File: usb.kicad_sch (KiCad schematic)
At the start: 8 parts, among them IC2 USB Hub, J2 2-Port USB, J3 2-Port USB

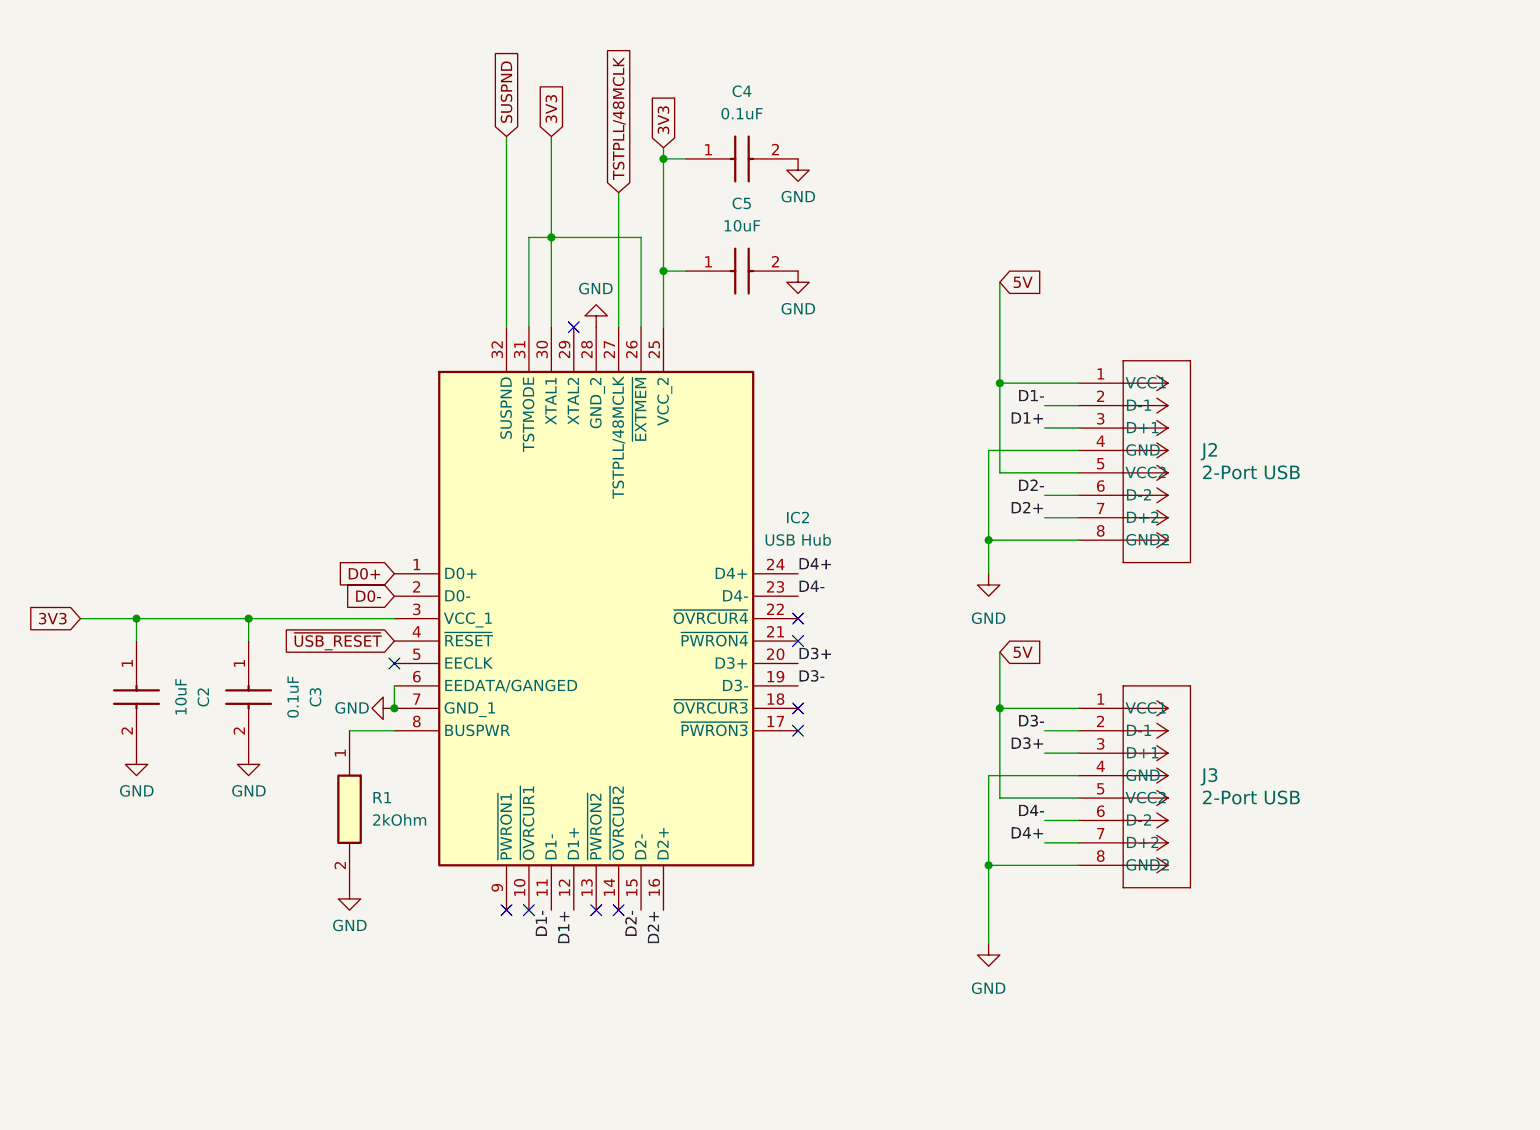
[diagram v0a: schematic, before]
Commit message: schematic fixes are done
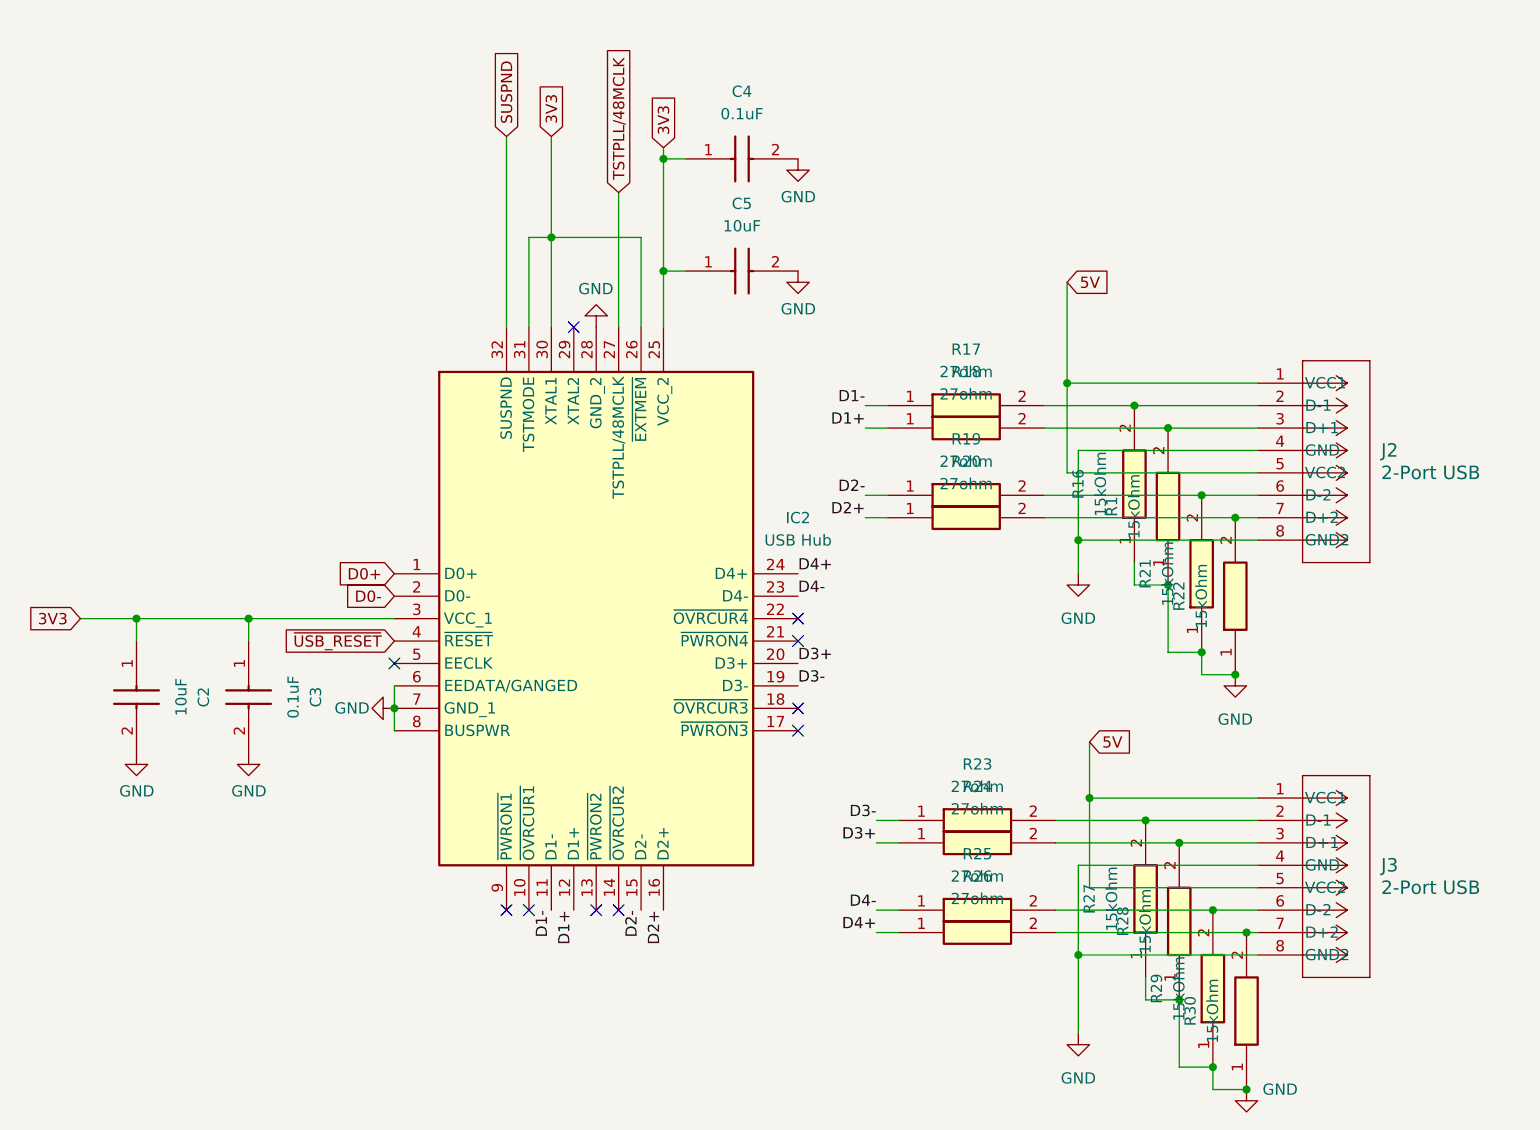
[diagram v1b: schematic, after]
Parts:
- added R16, R21, R22, R27, R28, R29, R30: 15kOhm, RESC2012X60N, symbol group127:Resistor
- added R17, R18, R19, R20, R23, R24, R25, R26: 27ohm, RESC2012X60N, symbol group127:Resistor
- R1: value 2kOhm -> 15kOhm; footprint Resistor_SMD:R_0805_2012Metric -> RESC2012X60N
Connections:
- net D1+: now also R18.1; no longer J2.3 (D+1)
- net D1-: now also R17.1; no longer J2.2 (D-1)
- net D2+: now also R20.1; no longer J2.7 (D+2)
- net D2-: now also R19.1; no longer J2.6 (D-2)
- net D3+: now also R24.1; no longer J3.3 (D+1)
- net D3-: now also R23.1; no longer J3.2 (D-1)
- net D4+: now also R26.1; no longer J3.7 (D+2)
- net D4-: now also R25.1; no longer J3.6 (D-2)
- net GND: now also IC2.8 (BUSPWR), R1.1, R16.1, R21.1, R22.1, R27.1, R28.1, R29.1, R30.1; no longer R1.2
- new net: J3.3 (D+1), R24.2, R28.2
- new net: J3.2 (D-1), R23.2, R27.2
- new net: J3.6 (D-2), R25.2, R29.2
- new net: J3.7 (D+2), R26.2, R30.2
- new net: J2.2 (D-1), R16.2, R17.2
- new net: J2.3 (D+1), R1.2, R18.2
- new net: J2.6 (D-2), R19.2, R21.2
- new net: J2.7 (D+2), R20.2, R22.2
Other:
- moved on the sheet: J2, J3
